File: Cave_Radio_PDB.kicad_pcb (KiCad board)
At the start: 2 copper layers, 53 x 37.8 mm, 85 parts, among them J1 Conn_01x02, J5 Conn_01x03, J6 Conn_01x02, J7 Conn_01x02, J8 Conn_01x02, J9 USB4110GFA, U1 TPS25751D, U2 CAT24C256, U3 TLV75533PDRV, U4 TVS2200DRV, U5 TPD2E2U06DRL, U6 LMR51450FNDRR, U7 LMR51450FNDRR, U8 TPS259472LRPWR, U9 NSR0340HT1G

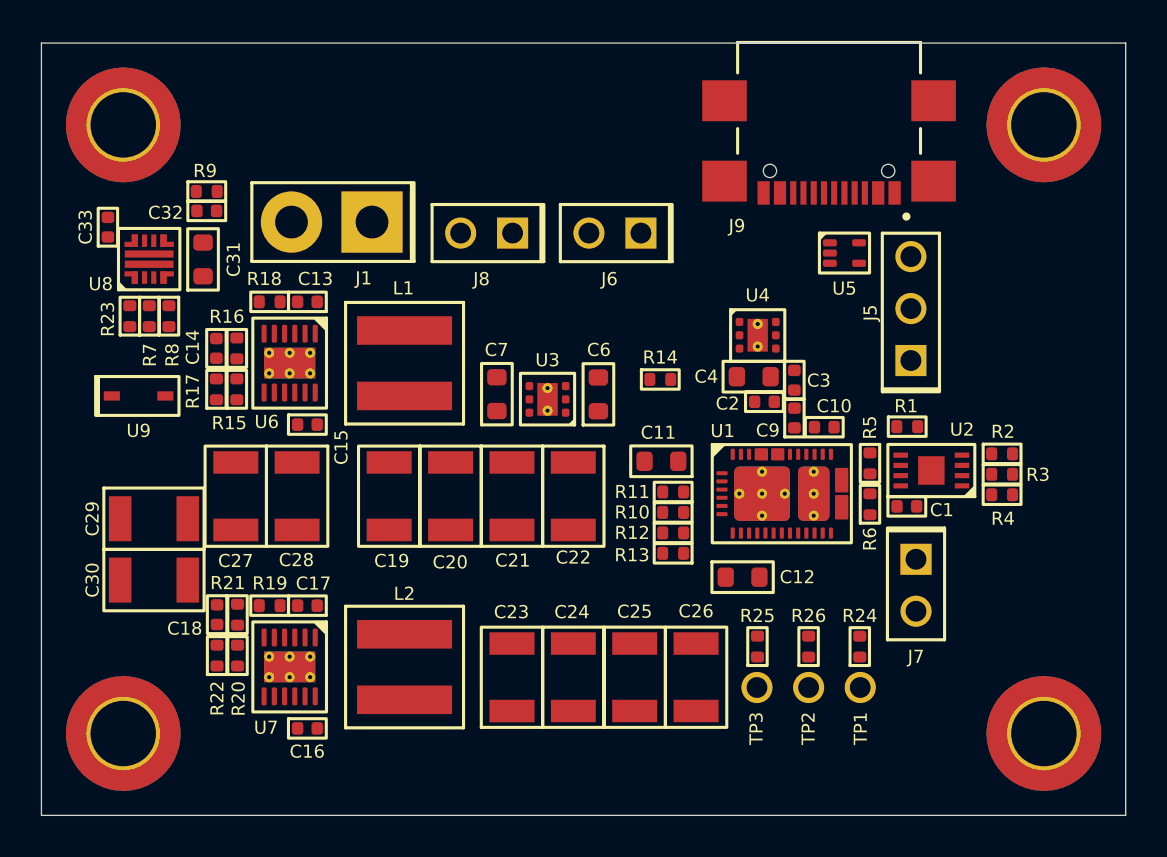
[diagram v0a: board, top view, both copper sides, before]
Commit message: initial layout
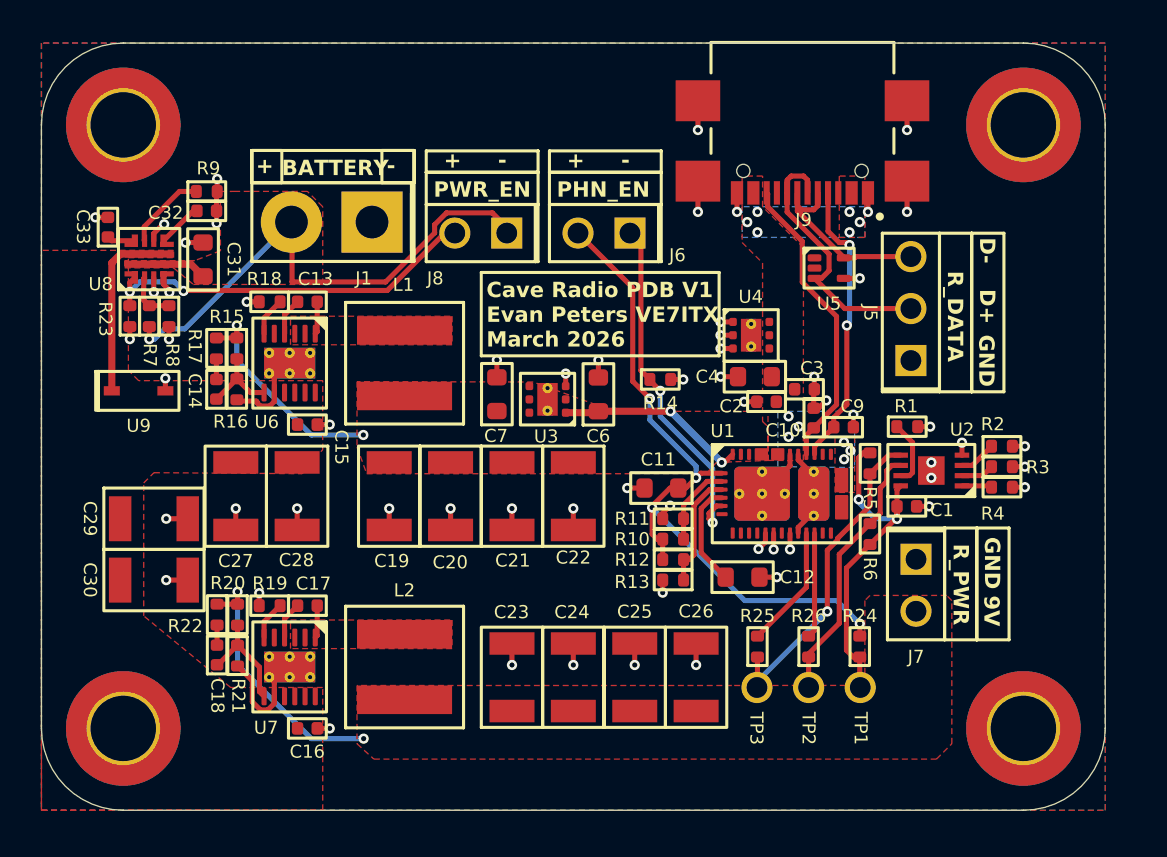
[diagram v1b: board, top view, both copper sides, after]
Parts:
- moved C9 2.44 mm to (130.2, 74.0), turned to 0 degrees
- moved R22 2.00 mm to (99.6, 83.2), turned to -90 degrees
- moved R17 2.00 mm to (99.6, 70.2), turned to -90 degrees
- moved R15 2.00 mm to (100.6, 70.2), turned to -90 degrees
- moved R16 2.00 mm to (100.6, 72.2), turned to -90 degrees
- moved R20 2.00 mm to (100.6, 83.2), turned to -90 degrees
- moved R21 2.00 mm to (100.6, 85.2), turned to -90 degrees
- moved C14 2.00 mm to (99.6, 72.2), turned to 90 degrees
- moved C18 1.97 mm to (99.6, 85.2), turned to 90 degrees
- moved R6 1.46 mm to (131.5, 79.2)
- moved H8 1.32 mm to (140.2, 84.5)
- moved C11 1.31 mm to (121.3, 77.0)
- moved R10 1.31 mm to (121.9, 79.5)
- moved R11 1.31 mm to (121.9, 78.5)
- moved R12 1.31 mm to (121.9, 80.5)
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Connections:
- J5 pad 1: /USB/D+ -> GND
- J5 pad 2: /USB/D- -> /USB/D+
- J5 pad 3: GND -> /USB/D-
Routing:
- net GND: track 0.00 -> 60.7 mm, vias 0 -> 60
- net LDO_3V3: track 0.00 -> 34.5 mm, vias 0 -> 4
- net Net-(J1-Pin_2): track 0.00 -> 28.6 mm, vias 0 -> 1
- net Net-(J8-Pin_2): track 0.00 -> 19.2 mm, vias 0 -> 2
- net 3V3_EEPROM: track 0.00 -> 17.1 mm, vias 0 -> 2
- net /USB/PD_EN: track 0.00 -> 16.9 mm, vias 0 -> 2
- net Net-(TP3-Pin_1): track 0.00 -> 16.1 mm, vias 0 -> 1
- net /USB/CC2: track 0.00 -> 14.8 mm
- net /USB/CC1: track 0.00 -> 14.1 mm, vias 0 -> 2
- net /USB/D+: track 0.00 -> 13.3 mm
- net Net-(TP2-Pin_1): track 0.00 -> 13.0 mm
- net 9V: track 0.00 -> 12.8 mm, vias 0 -> 2
- net 5V: track 0.00 -> 11.0 mm, vias 0 -> 2
- net /USB/D-: track 0.00 -> 9.84 mm
- net 3V3: track 0.00 -> 9.40 mm, vias 0 -> 2
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- added copper zone on F.Cu, net 5V
- added copper zone on F.Cu, net 9V
- added copper zone on B.Cu, net GND
- added copper zone on F.Cu, net GND
- added copper zone on F.Cu, net Net-(C13-Pad1)
- added copper zone on F.Cu, net Net-(C17-Pad1)
- added copper zone on F.Cu, net Net-(J1-Pin_2)
- added copper zone on F.Cu, net VBATT
- added copper zone on B.Cu, net VBUS
- added copper zone on F.Cu, net VBUS
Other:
- board size 53 x 37.8 mm -> 52 x 37.5 mm
- board text added: "+"
- board text added: "-"
- board text added: "9V"
- board text added: "BATTERY"
- board text added: "Cave Radio PDB V1 Evan Peters VE7ITX March 2026"
- board text added: "D+"
- board text added: "D-"
- board text added: "GND"
- board text added: "PHN_EN"
- board text added: "PWR_EN"
- board text added: "R_DATA"
- board text added: "R_PWR"
